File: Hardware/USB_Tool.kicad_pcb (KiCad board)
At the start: 2 copper layers, 100 x 77 mm, 49 parts, among them J1 USB_B_Micro, J2 CONN_ICSP, P1 TLMS1000, P2 150141M173100, P3 Green, P4 Green, SW1 SW_2TO1, U1 MRF89XAM8A, U2 NCP114, U3 MCP2210, U4 PIC18F46K40_44, X1 EXTENDER_SPI_1, X2 EXTENDER_IO_1, X3 EXTENDER_IO_2, X4 EXTENDER_POWER_2, X5 EXTENDER_POWER_2, X7 Extender_I2C_1, X8 Extender_I2C_2, X9 Extender_I2C_3, Y1 DSC6003JI2A

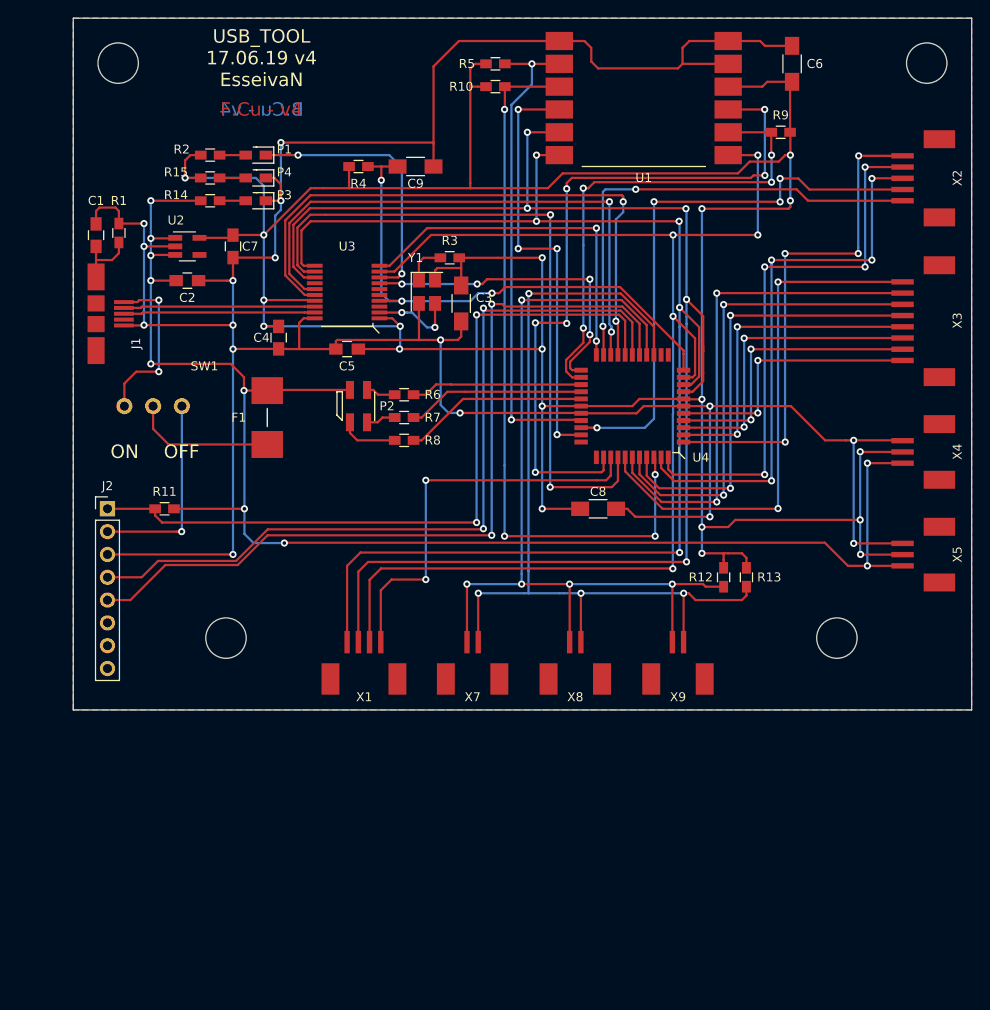
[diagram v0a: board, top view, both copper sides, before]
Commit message: v4 updated
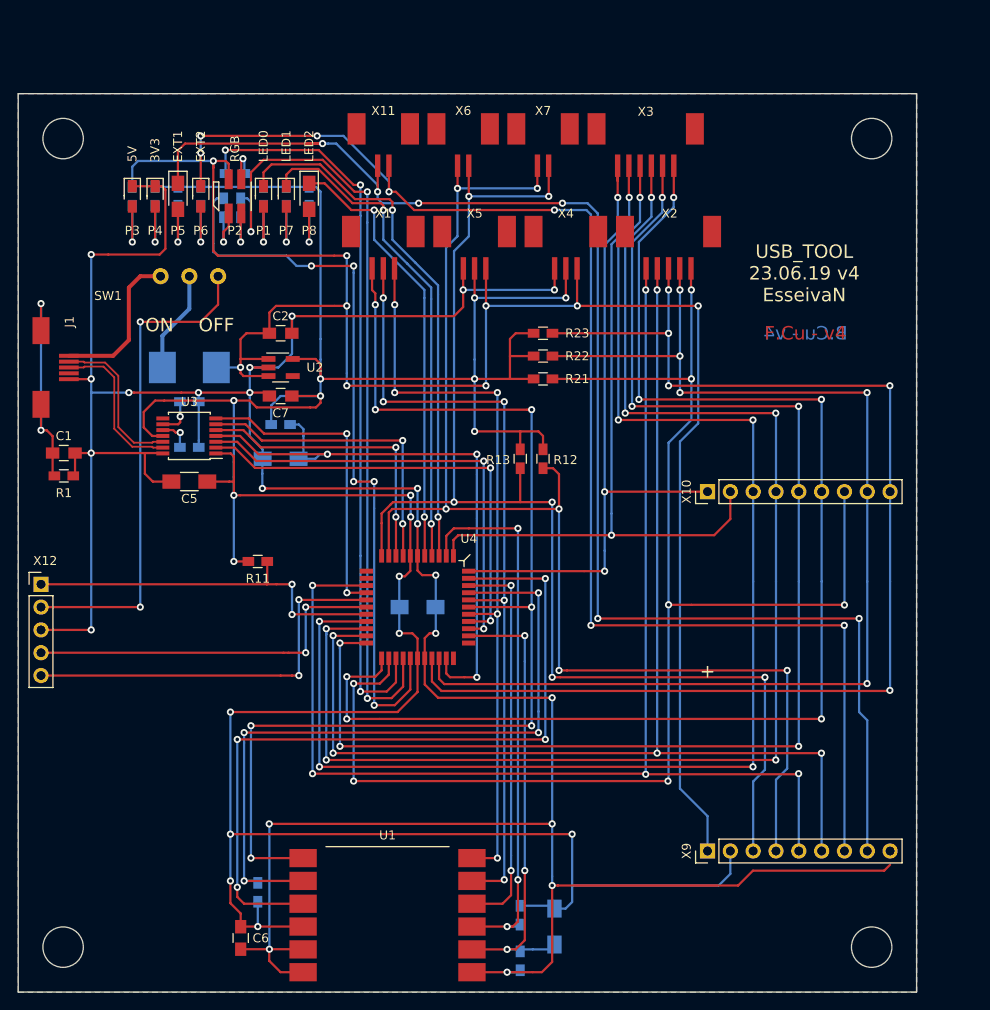
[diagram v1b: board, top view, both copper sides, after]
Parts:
- removed C4: 1uF, 0EsseivaN_Lib:C_0805_HandSoldering
- removed J2: CONN_ICSP, 0EsseivaN_Lib:Pin_Header_Straight_1x08_Pitch2.54mm
- removed the PERC-4.5mm at (61.1, 46.6)
- removed the PERC-4.5mm at (151.1, 46.6)
- removed the PERC-4.5mm at (141.1, 110.6)
- removed the PERC-4.5mm at (73.1, 110.6)
- removed X8: Extender_I2C_2, 0EsseivaN_Lib:CH_02P
- removed Y1: DSC6003JI2A, 0EsseivaN_Lib:Oscillator_SMD_4pin_2.5x2.0mm_HandSoldering
- added P5: Blue, 0EsseivaN_Lib:D_0805_HandSoldering, F.Cu at (67.8, 61.4)
- added P6: Green, 0EsseivaN_Lib:D_0603_HandSoldering, F.Cu at (70.3, 61.4)
- added P7: Green, 0EsseivaN_Lib:D_0603_HandSoldering, F.Cu at (79.8, 61.4)
- added P8: Blue, 0EsseivaN_Lib:D_0805_HandSoldering, F.Cu at (82.4, 61.4)
- added PERC-4.5mm: ~, 0EsseivaN_Lib:PERC-4.5mm, F.Cu at (55.0, 55.0)
- added PERC-4.5mm: ~, 0EsseivaN_Lib:PERC-4.5mm, F.Cu at (145.0, 55.0)
- added PERC-4.5mm: ~, 0EsseivaN_Lib:PERC-4.5mm, F.Cu at (55.0, 145.0)
- added PERC-4.5mm: ~, 0EsseivaN_Lib:PERC-4.5mm, F.Cu at (145.0, 145.0)
- added R16: 120R, 0EsseivaN_Lib:R_0603_HandSoldering, B.Cu at (67.8, 61.4)
- added R17: 270R, 0EsseivaN_Lib:R_0603_HandSoldering, B.Cu at (70.3, 61.4)
- added R18: 150R, 0EsseivaN_Lib:R_0603_HandSoldering, B.Cu at (79.8, 61.4)
- added R19: 4k7, 0EsseivaN_Lib:R_0603_HandSoldering, B.Cu at (69.0, 84.3)
- added R20: 4k7, 0EsseivaN_Lib:R_0603_HandSoldering, B.Cu at (69.0, 89.4)
- added R21: 4k7, 0EsseivaN_Lib:R_0603_HandSoldering, F.Cu at (108.4, 81.8)
- added R22: 4k7, 0EsseivaN_Lib:R_0603_HandSoldering, F.Cu at (108.4, 79.2)
- added R23: 4k7, 0EsseivaN_Lib:R_0603_HandSoldering, F.Cu at (108.4, 76.7)
- added X10: Extension, 0EsseivaN_Lib:Pin_Header_Straight_1x09_Pitch2.54mm, F.Cu at (126.7, 94.3)
- added X11: EXTENDER_LED_1, 0EsseivaN_Lib:CH_02P, F.Cu at (90.6, 57.6)
- added X12: CONN_ICSP, 0EsseivaN_Lib:Pin_Header_Straight_1x05_Pitch2.54mm, F.Cu at (52.5, 104.6)
- added X6: Extender_I2C_1, 0EsseivaN_Lib:CH_02P, F.Cu at (99.5, 57.6)
- C3, C8, C9, F1, R14, R15, R2, R4: moved to B.Cu
- C5: value 470nF -> 100nF; footprint 0EsseivaN_Lib:C_0805_HandSoldering -> 0EsseivaN_Lib:C_1206_HandSoldering
- C6: footprint 0EsseivaN_Lib:C_1206_HandSoldering -> 0EsseivaN_Lib:C_0805_HandSoldering
- P1: value TLMS1000 -> RED
- P2: value 150141M173100 -> RGB
- R10, R5, R9: value 1k -> 4k7; moved to B.Cu
- R12, R13: value 1k -> 4k7
- R3: value 1k -> 150R; moved to B.Cu
- R6, R7: value 180R -> 330R; moved to B.Cu
- R8: value 270R -> 560R; moved to B.Cu
- U3: value MCP2210 -> MCP2221A; footprint 0EsseivaN_Lib:SSOP-20_5.3x7.2mm_Pitch0.65mm -> 0EsseivaN_Lib:TSSOP-14_4.4x5mm_Pitch0.65mm
- X1: footprint 0EsseivaN_Lib:CH_04P -> 0EsseivaN_Lib:CH_03P
- X2: value EXTENDER_IO_1 -> EXTENDER_IO_2
- X3: value EXTENDER_IO_2 -> EXTENDER_IO_1; footprint 0EsseivaN_Lib:CH_08P -> 0EsseivaN_Lib:CH_06P
- X5: value EXTENDER_POWER_2 -> EXTENDER_POWER_1
- X7: value Extender_I2C_1 -> Extender_I2C_2
- X9: value Extender_I2C_3 -> Extension; footprint 0EsseivaN_Lib:CH_02P -> 0EsseivaN_Lib:Pin_Header_Straight_1x09_Pitch2.54mm
- moved C6 115.0 mm to (74.8, 144.0), turned to 270 degrees
- moved R9 102.7 mm to (76.7, 138.9), turned to 270 degrees
- moved R5 99.9 mm to (105.9, 146.5), turned to 90 degrees
- moved U1 95.3 mm to (91.1, 141.4), turned to 90 degrees
- moved R10 92.3 mm to (105.9, 141.4), turned to 90 degrees
- moved C3 70.1 mm to (109.7, 142.7)
- moved X5 58.6 mm to (100.8, 69.0), turned to 180 degrees
- moved X7 54.4 mm to (108.4, 57.6), turned to 180 degrees
- moved X4 43.8 mm to (111.0, 69.0), turned to 180 degrees
- moved X1 42.6 mm to (90.6, 69.0), turned to 180 degrees
- moved X3 36.4 mm to (119.8, 57.6), turned to 180 degrees
- moved C9 35.8 mm to (79.2, 90.6), turned to 180 degrees
- moved R8 32.8 mm to (72.9, 62.7), turned to 90 degrees
- moved U4 32.7 mm to (94.5, 107.2), turned to 270 degrees
- moved R6 31.0 mm to (74.1, 58.9), turned to 180 degrees
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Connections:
- net /CLK renamed /~INT1
- net /LED_B renamed /LEDRGB_B
- net /LED_G renamed /LEDRGB_G
- net /LED_R renamed /LEDRGB_R
- net VPP renamed /~MCLR
- C3 pad 2: GND -> /RESET_RF
- C9 pad 1: /RESET_USB -> /~RESET_USB
- J1 pad 2: D- -> /D-
- J1 pad 3: D+ -> /D+
- P1 pad 1: Net-(P1-Pad1) -> /LED0
- P1 pad 2: /SPI_LED -> Net-(P1-Pad2)
- P3 pad 1: Net-(P3-Pad1) -> GND
- P3 pad 2: GND -> Net-(P3-Pad2)
- P4 pad 1: Net-(P4-Pad1) -> GND
- P4 pad 2: GND -> Net-(P4-Pad2)
- R11 pad 1: 5V -> 3V3
- R12 pad 1: SDA -> /SCL
- R13 pad 1: SCL -> /SDA
- R14 pad 2: Net-(P3-Pad1) -> Net-(P3-Pad2)
- R15 pad 2: Net-(P4-Pad1) -> Net-(P4-Pad2)
- R2 pad 2: Net-(P1-Pad1) -> Net-(P8-Pad2)
- R3 pad 1: Net-(R3-Pad1) -> 3V3
- R3 pad 2: 3V3 -> Net-(P1-Pad2)
- R4 pad 1: /RESET_USB -> /~RESET_USB
- R5 pad 1: /RESET_RF -> GND
- R5 pad 2: 3V3 -> /RESET_RF
- SW1 pad 3: Net-(J2-Pad2) -> /ICSP_VCC
- U3 pad 10: /~LOWPWR -> Net-(R20-Pad2)
- U3 pad 11: /SCK -> 3V3
- U3 pad 12: /~USBCFG -> /D-
- U3 pad 13: /MOSI -> /D+
- U3 pad 14: Net-(U3-Pad14) -> GND
- U3 pad 2: Net-(U3-Pad2) -> /SSPND
- U3 pad 3: Net-(U3-Pad3) -> /USB_IOC
- U3 pad 4: /RESET_USB -> /~RESET_USB
- U3 pad 5: Net-(U3-Pad5) -> /Tx
- U3 pad 6: Net-(U3-Pad6) -> /Rx
- U3 pad 7: /~SSPND -> /USBCFG
- U3 pad 8: /SPI_LED -> Net-(U3-Pad8)
- U3 pad 9: /MISO -> Net-(R19-Pad2)
- U4 pad 1: /D3 -> /D1
- U4 pad 10: /MISO -> /SCL
- U4 pad 11: /RESET_USB -> /SDA
- U4 pad 14: SCL -> /CLKR
- U4 pad 15: SDA -> /USBCFG
- U4 pad 16: ICSPCLK -> /ICSPCLK
- U4 pad 17: ICSPDAT -> /ICSPDAT
- U4 pad 19: /BRR -> /D2
- U4 pad 2: /D8 -> /~CSCON
- U4 pad 20: /BRA -> /D3
- U4 pad 21: /INT -> /DAC_OUT
- U4 pad 22: /~LOWPWR -> /D4
- U4 pad 23: /~SSPND -> /D5
- U4 pad 24: /~CSDAT -> /~INT0
- U4 pad 3: /D9 -> /LED0
- U4 pad 30: /RESET_RF -> /~INT2
- U4 pad 32: /IRQ0 -> /~RESET_USB
- U4 pad 35: /IRQ1 -> /RESET_RF
- U4 pad 36: /CS_EXT -> /USB_IOC
- U4 pad 37: /~USBCFG -> /SSPND
- U4 pad 38: /D4 -> /SCK
- U4 pad 39: /D5 -> /MISO
- U4 pad 4: /D10 -> /LED1
- U4 pad 40: /D6 -> /MOSI
- U4 pad 41: /D7 -> /~CSDAT
- U4 pad 42: /~CSCON -> /IRQ0
- U4 pad 43: /D1 -> /IRQ1
- U4 pad 44: /D2 -> /D0
- U4 pad 5: /D11 -> /LED2
- U4 pad 8: /MOSI -> /Rx
- U4 pad 9: /SCK -> /Tx
- X2 pad 1: /INT -> /~INT0
- X2 pad 3: /D1 -> /~INT2
- X2 pad 4: /D2 -> /DAC_OUT
- X2 pad 5: /D3 -> /CLKR
- X3 pad 1: /D11 -> /D5
- X3 pad 2: /D10 -> /D4
- X3 pad 3: /D9 -> /D3
- X3 pad 4: /D8 -> /D2
- X3 pad 5: /D7 -> /D1
- X3 pad 6: /D6 -> /D0
- X7 pad 1: SDA -> /SDA
- X7 pad 2: SCL -> /SCL
- X9 pad 1: SDA -> 5V
- X9 pad 2: SCL -> 3V3
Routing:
- net Net-(P5-Pad1): track 0.00 -> 159.7 mm, vias 0 -> 6
- net /~INT0: track 0.00 -> 157.8 mm, vias 0 -> 7
- net Net-(P6-Pad1): track 0.00 -> 155.5 mm, vias 0 -> 7
- net /CLKR: track 0.00 -> 146.0 mm, vias 0 -> 5
- net /SCL: track 0.00 -> 144.0 mm, vias 0 -> 6
- net /SDA: track 0.00 -> 141.5 mm, vias 0 -> 6
- net /~INT2: track 0.00 -> 138.6 mm, vias 0 -> 5
- net /DAC_OUT: track 0.00 -> 136.0 mm, vias 0 -> 5
- net SCL: track 99.7 -> 0.00 mm, vias 4 -> 0
- net SDA: track 98.1 -> 0.00 mm, vias 5 -> 0
- net /D3: track 56.2 -> 153.6 mm, vias 4 -> 6
- net ICSPCLK: track 92.5 -> 0.00 mm, vias 2 -> 0
- net /D4: track 59.4 -> 150.5 mm, vias 2 -> 6
- net /D2: track 61.9 -> 152.6 mm, vias 4 -> 6
- net /D5: track 56.4 -> 146.6 mm, vias 2 -> 6
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- added copper zone on B.Cu, net 3V3
- removed copper zone on B.Cu, net 5V
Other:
- board size 100 x 77 mm -> 100 x 100 mm
- net class USB_Unprotected added: clearance 0.2, trace_width 0.45, via_dia 1, via_drill 0.6
- board text added: "+"
- board text added: "3V3"
- board text added: "5V"
- board text added: "EXT1"
- board text added: "EXT2"
- board text added: "LED0"
- board text added: "LED1"
- board text added: "LED2"
- board text added: "RGB"
- board text added: "USB_TOOL 23.06.19 v4 EsseivaN"
- board text added: "USB_TOOL 23.06.19 v4 Esseivan"
- board text removed: "USB_TOOL 17.06.19 v4 EsseivaN"
- board text removed: "USB_TOOL 17.06.19 v4 Esseivan"
